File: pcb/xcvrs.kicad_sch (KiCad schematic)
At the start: 12 parts, among them SW1 TermSw, U301 TCAN3403-Q1, U302 74LVC1G07, U303 SN74LV1T34DBV

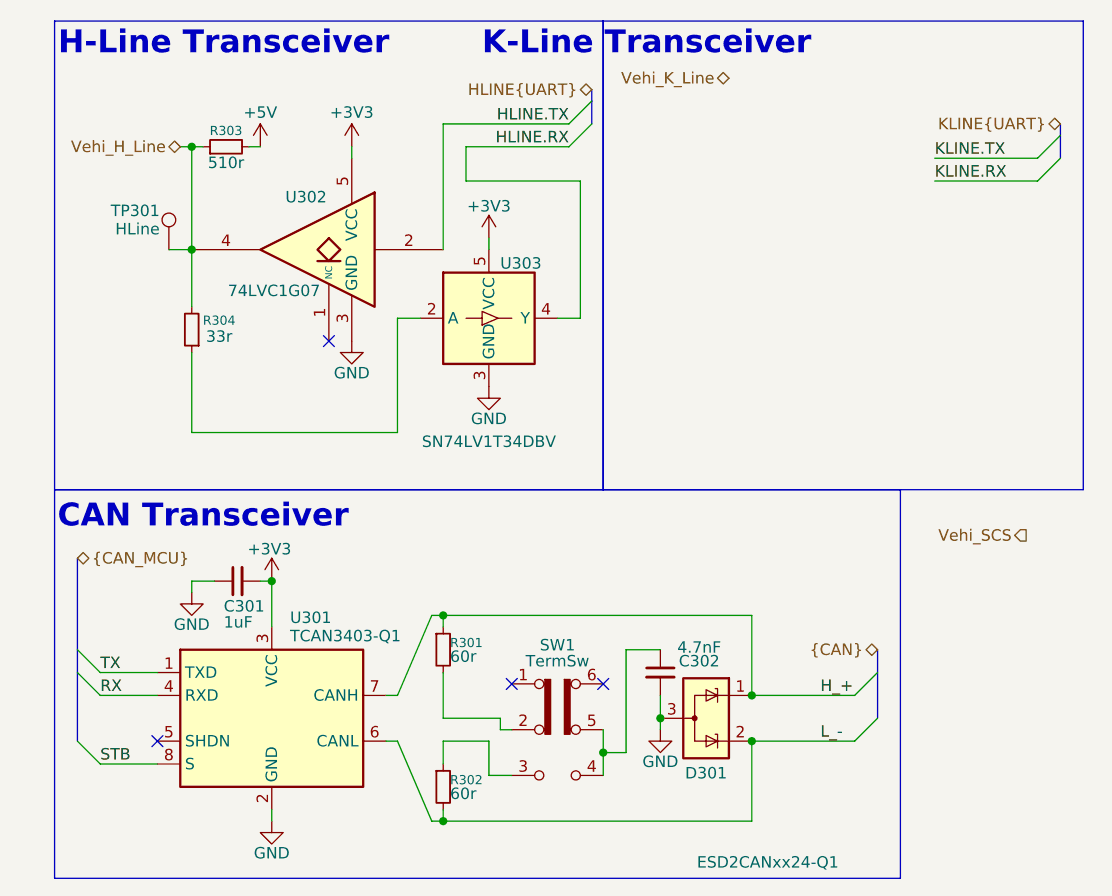
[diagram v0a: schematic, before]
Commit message: Add TLIN2027, placement, DRC fixes, routing
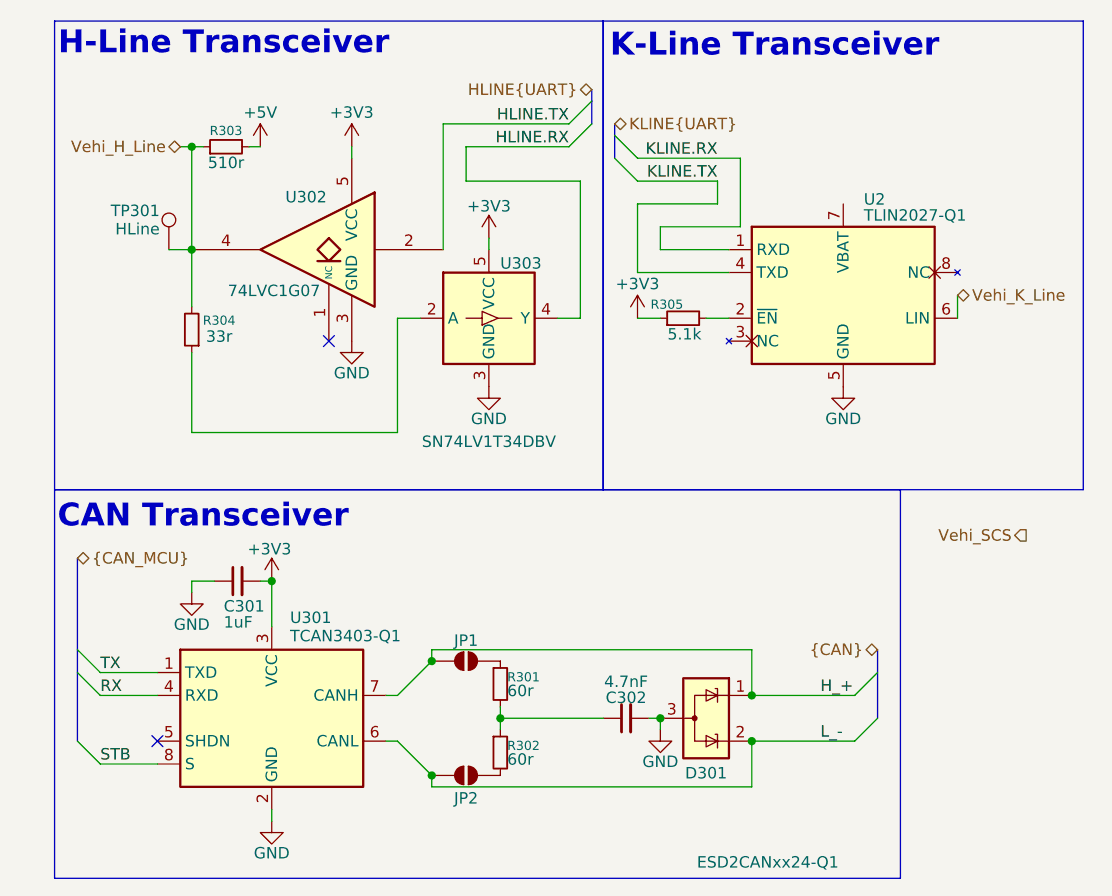
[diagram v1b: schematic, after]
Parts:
- removed SW1: TermSw, Button_Switch_SMD:SW_DPDT_CK_JS202011JCQN, symbol Switch:SW_Slide_DPDT
- added JP1, JP2: SolderJumper_2_Open, Jumper:SolderJumper-2_P1.3mm_Open_RoundedPad1.0x1.5mm, symbol Jumper:SolderJumper_2_Open
- added R305: 5.1k, Resistor_SMD:R_0402_1005Metric, symbol Device:R_Small
- added U2: TLIN2027-Q1, Package_SO:SOIC-8_3.9x4.9mm_P1.27mm, symbol TIParts:TLIN2027DRQ1
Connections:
- net +3V3: now also R305.1
- net GND: now also U2.5 (GND)
- net H_+: now also JP1.1 (A); no longer R301.1
- net KLINE.RX: now also U2.1 (RXD)
- net KLINE.TX: now also U2.4 (TXD)
- net L_-: now also JP2.2 (B); no longer R302.2
- net Vehi_K_Line: now also U2.6 (LIN)
- net at R301.2: now also C302.1, R302.1
- new net: JP2.1 (A), R302.2
- new net: JP1.2 (B), R301.1
- new net: R305.2, U2.2 (~{EN})
- no-connect marks 4 -> 2
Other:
- moved on the sheet: C302, R301, R302
